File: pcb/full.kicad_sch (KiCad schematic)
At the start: 118 parts, among them J1 MJ-4PP-9, J2 MJ-4PP-9, SW1 SW_PUSH, SW10 SW_PUSH, SW11 SW_PUSH, SW12 SW_PUSH, SW13 SW_PUSH, SW14 SW_PUSH, SW15 SW_PUSH, SW16 SW_PUSH, SW17 SW_PUSH, SW18 SW_PUSH, SW19 SW_PUSH, SW2 SW_PUSH, SW20 SW_PUSH, SW21 SW_PUSH, SW22 SW_PUSH, SW23 SW_PUSH, SW24 SW_PUSH, SW25 SW_PUSH, SW26 SW_PUSH, SW27 SW_PUSH, SW28 SW_PUSH, SW29 SW_PUSH, SW3 SW_PUSH, SW30 SW_PUSH, SW31 SW_PUSH, SW32 SW_PUSH, SW33 SW_PUSH, SW34 SW_PUSH, SW35 SW_PUSH, SW36 SW_PUSH, SW37 SW_PUSH, SW38 SW_PUSH, SW39 SW_PUSH, SW4 SW_PUSH, SW40 SW_PUSH, SW5 SW_PUSH, SW6 SW_PUSH, SW7 SW_PUSH, SW8 SW_PUSH, SW9 SW_PUSH, U1 xiao-ble, U2 xiao-ble

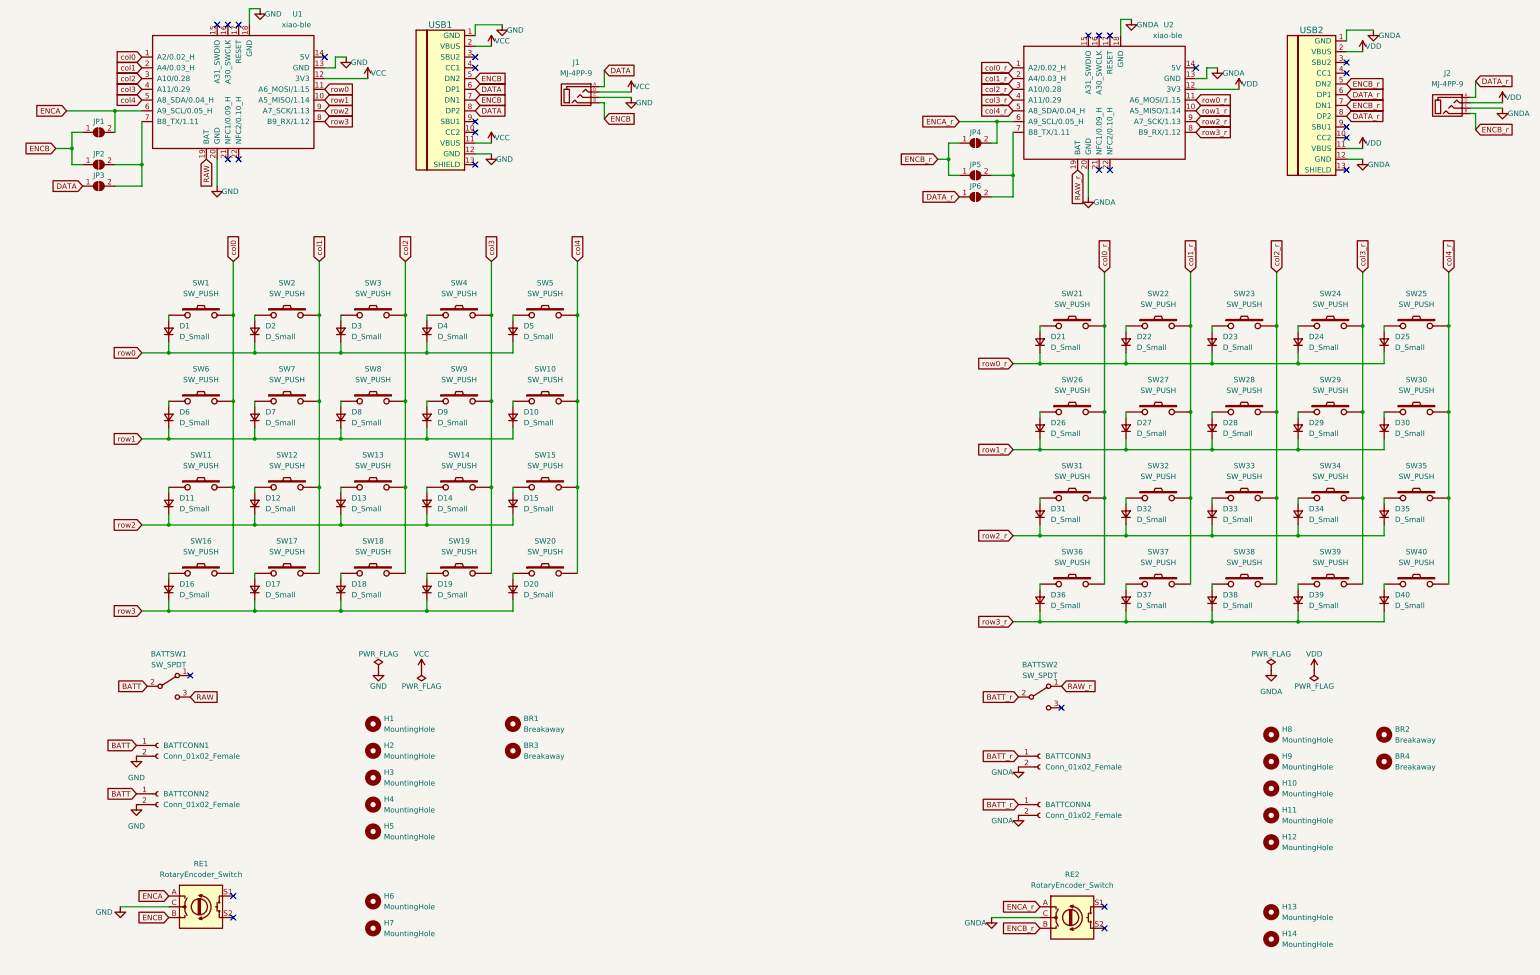
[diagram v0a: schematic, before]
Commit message: fix components and pcbs
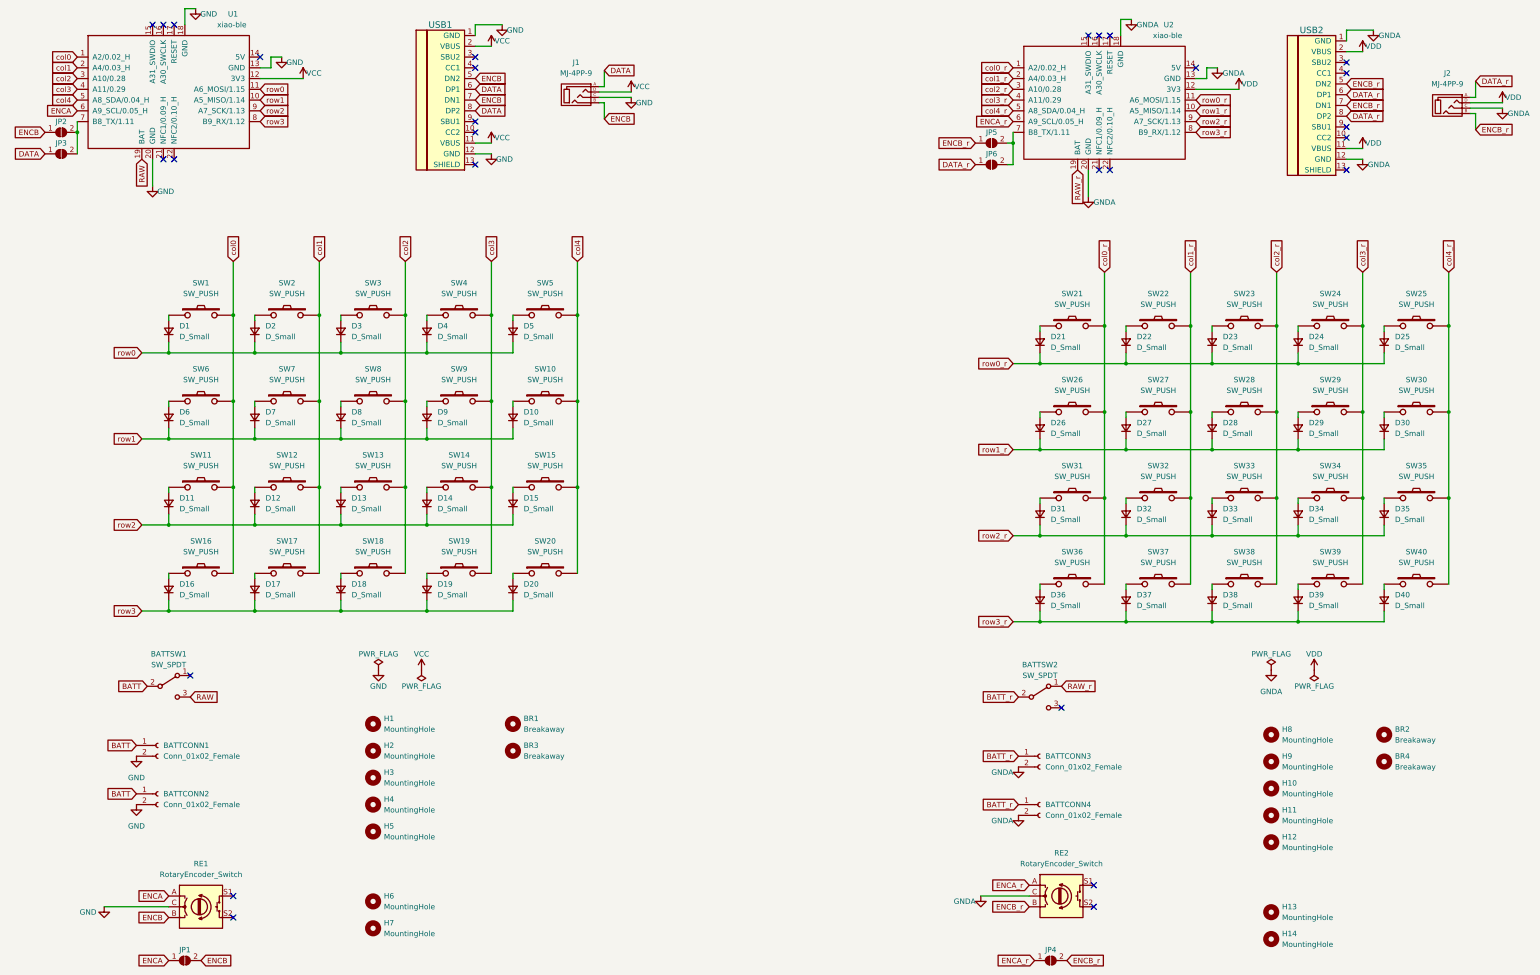
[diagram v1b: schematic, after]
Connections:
- net ENCA: now also JP1.1 (A); no longer JP1.2 (B)
- net ENCA_r: now also JP4.1 (A); no longer JP4.2 (B)
- net ENCB: now also JP1.2 (B); no longer JP1.1 (A)
- net ENCB_r: now also JP4.2 (B); no longer JP4.1 (A)
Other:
- moved on the sheet: JP1, JP2, JP3, JP4, JP5, JP6, RE2, U1
